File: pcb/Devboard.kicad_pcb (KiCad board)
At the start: 2 copper layers, 22.2 x 52.2 mm, 36 parts, among them J1 USB_C_Receptacle_USB2.0_14P, J2 Conn_01x20, J3 Conn_01x20, J4 Conn_01x03, SW1 SW_Push, U1 RP2040, U2 NCP1117-3.3_SOT223, U3 W25Q128JVS, Y1 12 MHz

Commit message: added bom
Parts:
- C1, C11, C12, C17, C3, C4, C5, C6, C7, C8, C9: value C -> .1uF
- C10, C2: value C -> 1uF
- C13, C14: value C -> 10uF
- R2, R7: value R -> 1K
- R4, R5: value R -> 27
- R6: value R -> 10K
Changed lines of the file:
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@@
 			(outputformat 1)
 			(mirror no)
-			(drillshape 1)
+			(drillshape 0)
 			(scaleselection 1)
-			(outputdirectory "")
+			(outputdirectory "C:/Users/aarus/OneDrive/Documents/Devboard/production/")
 		)
 	)
@@
 			)
 		)
-		(property "Value" "C"
+		(property "Value" ".1uF"
 			(at 0 1.16 90)
 			(layer "F.Fab")
@@
 			)
 		)
-		(property "Value" "C"
+		(property "Value" ".1uF"
 			(at 0 1.16 0)
 			(layer "F.Fab")
@@
 			)
 		)
-		(property "Value" "C"
+		(property "Value" ".1uF"
 			(at 0 1.16 0)
 			(layer "F.Fab")
@@
 			)
 		)
-		(property "Value" "C"
+		(property "Value" ".1uF"
 			(at 0 1.16 0)
 			(layer "F.Fab")
@@
 			)
 		)
-		(property "Value" "C"
+		(property "Value" ".1uF"
 			(at 0 1.16 90)
 			(layer "F.Fab")
@@
 			)
 		)
-		(property "Value" "C"
+		(property "Value" ".1uF"
 			(at 0 1.16 0)
 			(layer "F.Fab")
@@
 			)
 		)
-		(property "Value" "C"
+		(property "Value" "1uF"
 			(at 0 1.16 90)
 			(layer "F.Fab")
@@
 			)
 		)
-		(property "Value" "C"
+		(property "Value" ".1uF"
 			(at 0 1.16 90)
 			(layer "F.Fab")
@@
 			)
 		)
-		(property "Value" "R"
+		(property "Value" "1K"
 			(at 0 1.17 90)
 			(layer "F.Fab")
@@
 			)
 		)
-		(property "Value" "R"
+		(property "Value" "1K"
 			(at 0 1.17 90)
 			(layer "F.Fab")
@@
 			)
 		)
-		(property "Value" "C"
+		(property "Value" "10uF"
 			(at 0 1.16 0)
 			(layer "F.Fab")
@@
 			)
 		)
-		(property "Value" "R"
+		(property "Value" "27"
 			(at 0 1.17 90)
 			(layer "F.Fab")
@@
 			)
 		)
-		(property "Value" "C"
+		(property "Value" ".1uF"
 			(at 0 1.16 90)
 			(layer "F.Fab")
@@
 			)
 		)
-		(property "Value" "C"
+		(property "Value" ".1uF"
 			(at 0 1.16 0)
 			(layer "F.Fab")
@@
 			)
 		)
-		(property "Value" "C"
+		(property "Value" "1uF"
 			(at 0 1.16 90)
 			(layer "F.Fab")
@@
 			)
 		)
-		(property "Value" "R"
+		(property "Value" "27"
 			(at 0 1.17 0)
 			(layer "F.Fab")
@@
 			)
 		)
-		(property "Value" "C"
+		(property "Value" ".1uF"
 			(at 0 1.16 0)
 			(layer "F.Fab")
@@
 			)
 		)
-		(property "Value" "C"
+		(property "Value" "10uF"
 			(at 0 1.16 0)
 			(layer "F.Fab")
@@
 			)
 		)
-		(property "Value" "C"
+		(property "Value" ".1uF"
 			(at 0 1.16 0)
 			(layer "F.Fab")
@@
 			)
 		)
-		(property "Value" "R"
+		(property "Value" "10K"
 			(at 0 1.452578 0)
 			(layer "F.Fab")

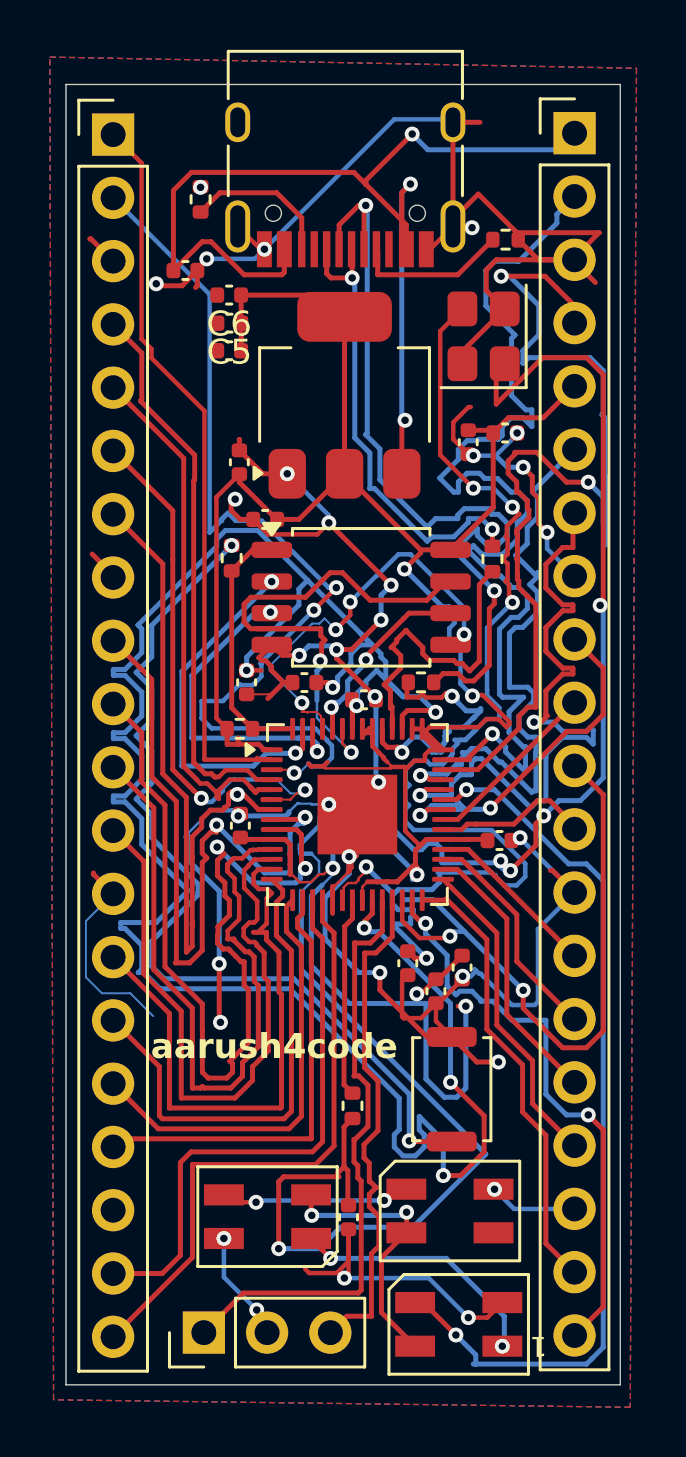
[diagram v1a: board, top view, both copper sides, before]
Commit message: updated routing
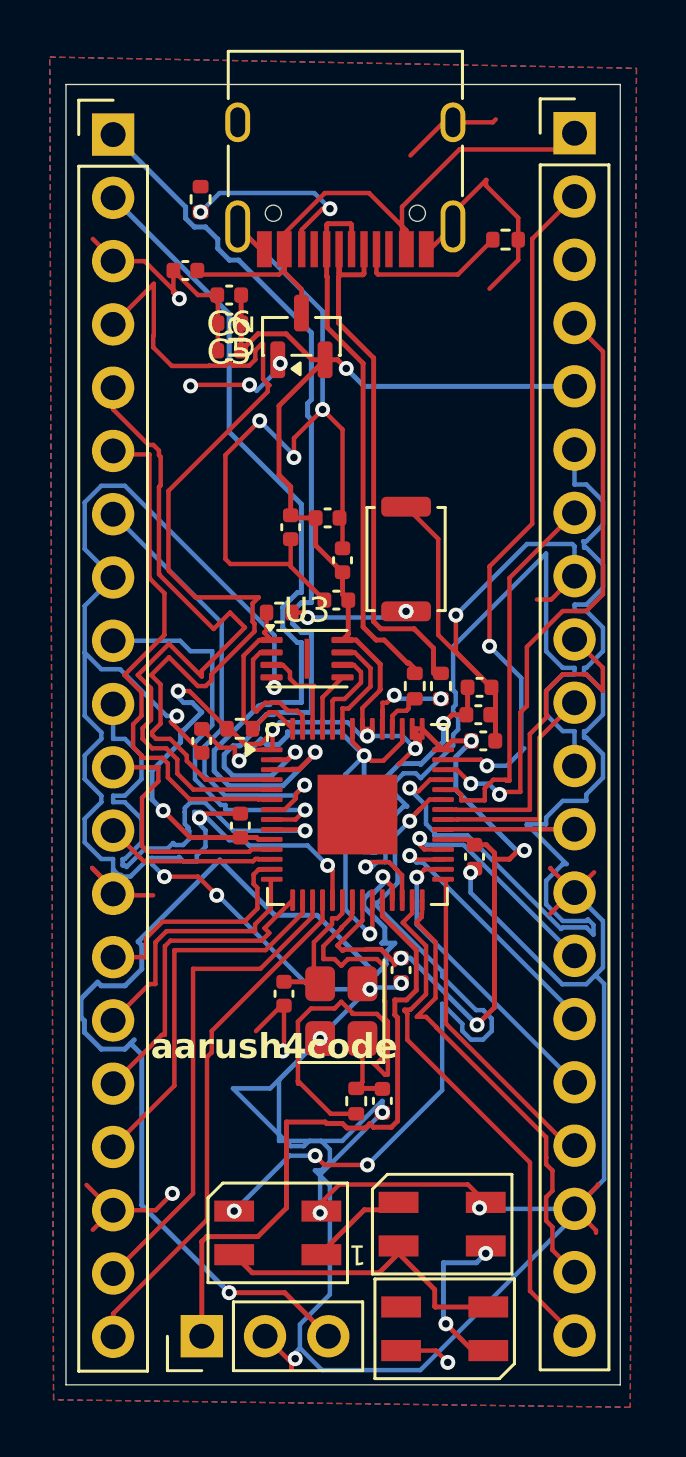
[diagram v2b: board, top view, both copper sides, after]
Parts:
- U2: value NCP1117-3.3_SOT223 -> MCP1700x-330xxTT; footprint Package_TO_SOT_SMD:SOT-223-3_TabPin2 -> Package_TO_SOT_SMD:SOT-23
- U3: value W25Q128JVS -> W25Q16JVSS; footprint Package_SO:SOIC-8_5.3x5.3mm_P1.27mm -> Package_SON:Winbond_USON-8-1EP_3x2mm_P0.5mm_EP0.2x1.6mm
- moved Y1 27.7 mm to (210.8, 97.2)
- moved SW1 21.4 mm to (213.4, 79.0)
- moved D1 8.14 mm to (208.2, 106.1)
- moved C13 7.90 mm to (210.2, 77.4)
- moved C17 7.90 mm to (208.8, 77.8)
- moved C11 7.03 mm to (216.3, 84.2), turned to 0 degrees
- moved D2 7.02 mm to (214.8, 105.8), turned to 180 degrees
- moved R5 5.98 mm to (213.8, 84.2)
- moved C1 5.71 mm to (210.8, 79.1)
- moved C2 5.62 mm to (216.2, 91.0)
- moved C15 5.12 mm to (208.5, 96.5)
- moved C16 4.87 mm to (212.4, 100.8)
- moved D3 4.73 mm to (214.9, 110.0), turned to 0 degrees
- moved C12 4.63 mm to (216.3, 85.3)
- moved C8 4.32 mm to (210.6, 80.7)
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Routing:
- net GND: track 181.4 -> 265.2 mm, vias 32 -> 25
- net Net-(C16-Pad2): track 78.0 -> 3.73 mm, vias 5 -> 0
- net +1V1: track 92.1 -> 35.0 mm, vias 7 -> 4
- net XIN: track 49.3 -> 5.54 mm, vias 5 -> 0
- net Net-(R7-Pad1): track 37.4 -> 4.77 mm
- net SWD: track 20.5 -> 44.0 mm, vias 0 -> 2
- net +3V3: track 116.8 -> 93.5 mm, vias 6 -> 10
- net VBUS: track 45.7 -> 24.8 mm, vias 3 -> 0
- net GPIO9: track 26.1 -> 6.93 mm
- net GPIO8: track 28.8 -> 10.6 mm
- net GPIO2: track 23.0 -> 41.1 mm
- net QPSI_SD3: track 22.1 -> 4.43 mm, vias 2 -> 0
- net GPIO28_ADC2: track 41.1 -> 24.8 mm
- net GPIO27_ADC1: track 25.0 -> 40.9 mm
- net GPIO29_ADC3: track 43.4 -> 27.9 mm, vias 1 -> 2
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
